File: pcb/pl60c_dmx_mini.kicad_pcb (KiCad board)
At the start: 4 copper layers, 38.5 x 29 mm, 36 parts, among them J1 USB-C 16P, J2 XLR-5 female (DMX OUT), Q1 S8050, SW2 BOOT, SW3 USER, U1 ESP32-S3-MINI-1-N8, U2 AP2112K-3.3, U3 SP3485EN, U4 USBLC6-2SC6

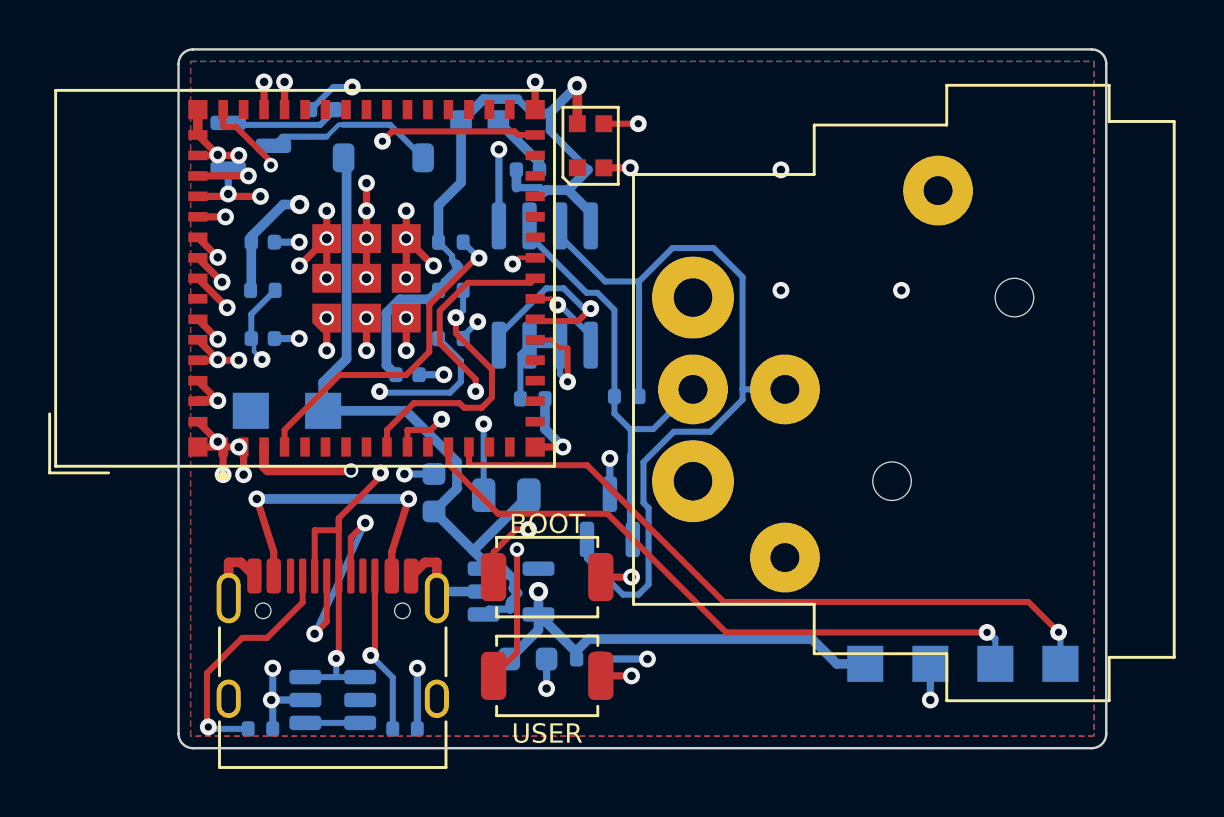
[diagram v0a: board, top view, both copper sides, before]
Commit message: auto: 2026-09-02 14:24:11
Co-Authored-By: Claude Fable 5.1 <noreply@anthropic.com>
Claude-Session: https://claude.ai/code/session_01WsrVZb94LwbHVAmBvsSTfn
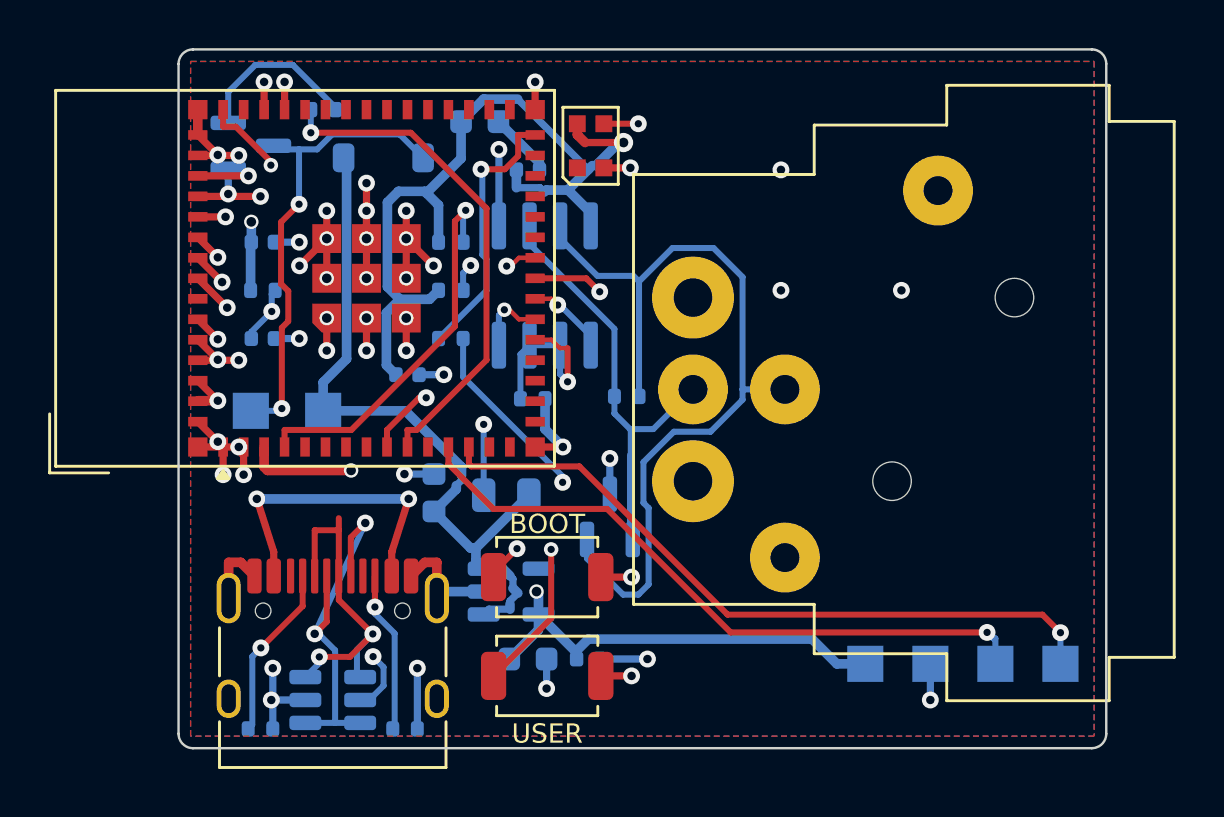
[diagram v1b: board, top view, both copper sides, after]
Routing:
- net BZ_N: track 7.14 -> 19.6 mm, vias 0 -> 2
- net LED_DATA_R: track 15.1 -> 26.6 mm
- net LED_DATA: track 22.8 -> 11.3 mm, vias 2 -> 1
- net VBUS: track 20.3 -> 31.4 mm, vias 3 -> 4
- net USB_D-: track 29.1 -> 39.5 mm
- net USB_D+: track 40.4 -> 33.0 mm
- net +3V3: track 97.0 -> 104.3 mm
- net DMX_TX: track 7.93 -> 3.01 mm
- net IO0_BOOT: track 28.8 -> 32.9 mm
- net EN: track 15.4 -> 12.1 mm
- net CC1: track 10.2 -> 7.28 mm
- net Q1_B: track 4.74 -> 7.02 mm
- net BUZZER: track 20.6 -> 21.0 mm, vias 2 -> 1
- net BTN_USER: track 27.5 -> 27.6 mm, vias 2 -> 3

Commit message: auto: 2026-09-02 14:26:12
Co-Authored-By: Claude Fable 5.1 <noreply@anthropic.com>
Claude-Session: https://claude.ai/code/session_01WsrVZb94LwbHVAmBvsSTfn
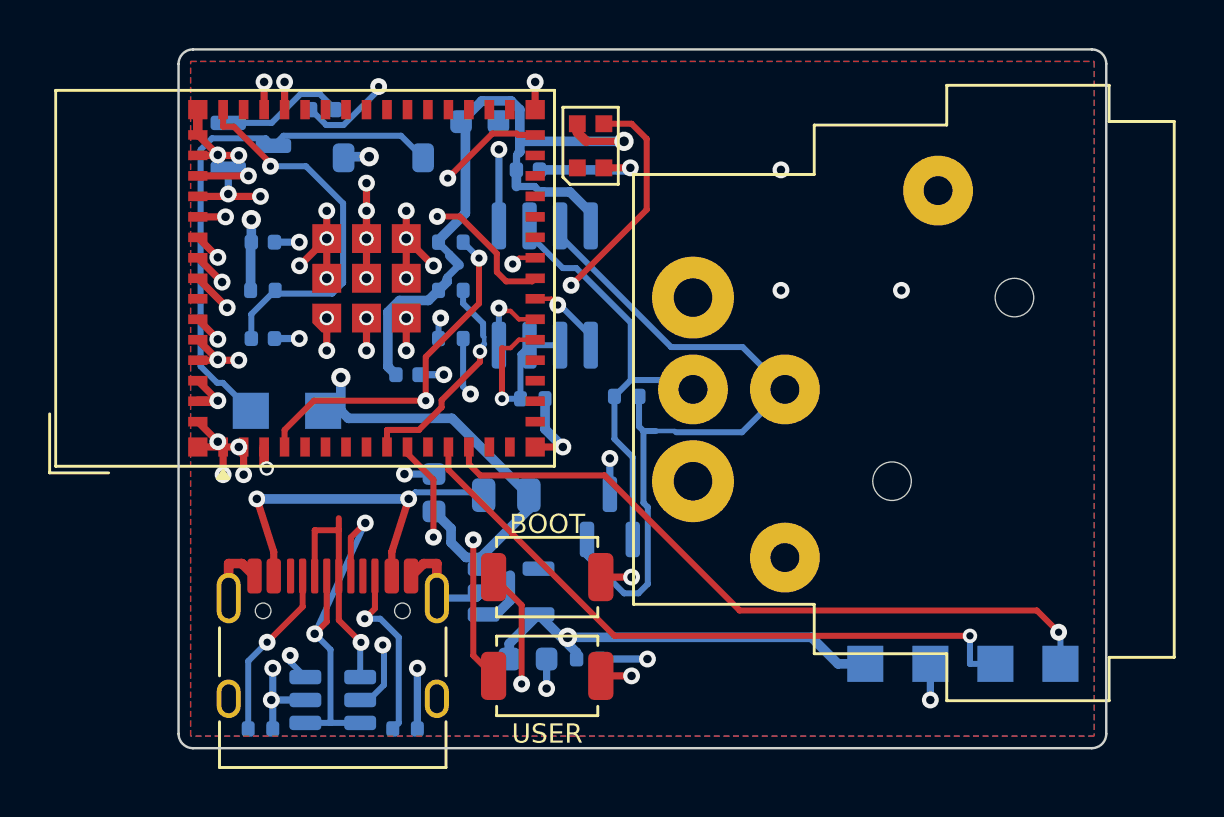
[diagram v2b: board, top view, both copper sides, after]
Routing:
- net USB_D+: track 33.0 -> 48.2 mm
- net BUZZER: track 21.0 -> 29.5 mm, vias 1 -> 2
- net VBUS: track 31.4 -> 25.7 mm, vias 4 -> 3
- net DMX_B: track 36.0 -> 31.0 mm
- net LED_DATA_R: track 26.6 -> 22.1 mm
- net BTN_USER: track 27.6 -> 23.5 mm, vias 3 -> 2
- net EN: track 12.1 -> 15.8 mm, vias 2 -> 1
- net BZ_N: track 19.6 -> 21.9 mm, vias 2 -> 0
- net +5V: track 30.5 -> 32.8 mm, vias 0 -> 2
- net Q1_B: track 7.02 -> 5.21 mm
- net GND: track 85.4 -> 86.3 mm
- net CC2: track 6.72 -> 7.58 mm
- net IO0_BOOT: track 32.9 -> 33.2 mm, vias 2 -> 3
- net LED_DATA: track 11.3 -> 11.4 mm, vias 1 -> 2
